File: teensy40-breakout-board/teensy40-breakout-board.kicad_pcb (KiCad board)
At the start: 2 copper layers, 18 x 56.1 mm, 3 parts, among them J1 Conn_01x08, J2 Conn_01x08, U1 Teensy4.0_WithBottomAndEdge

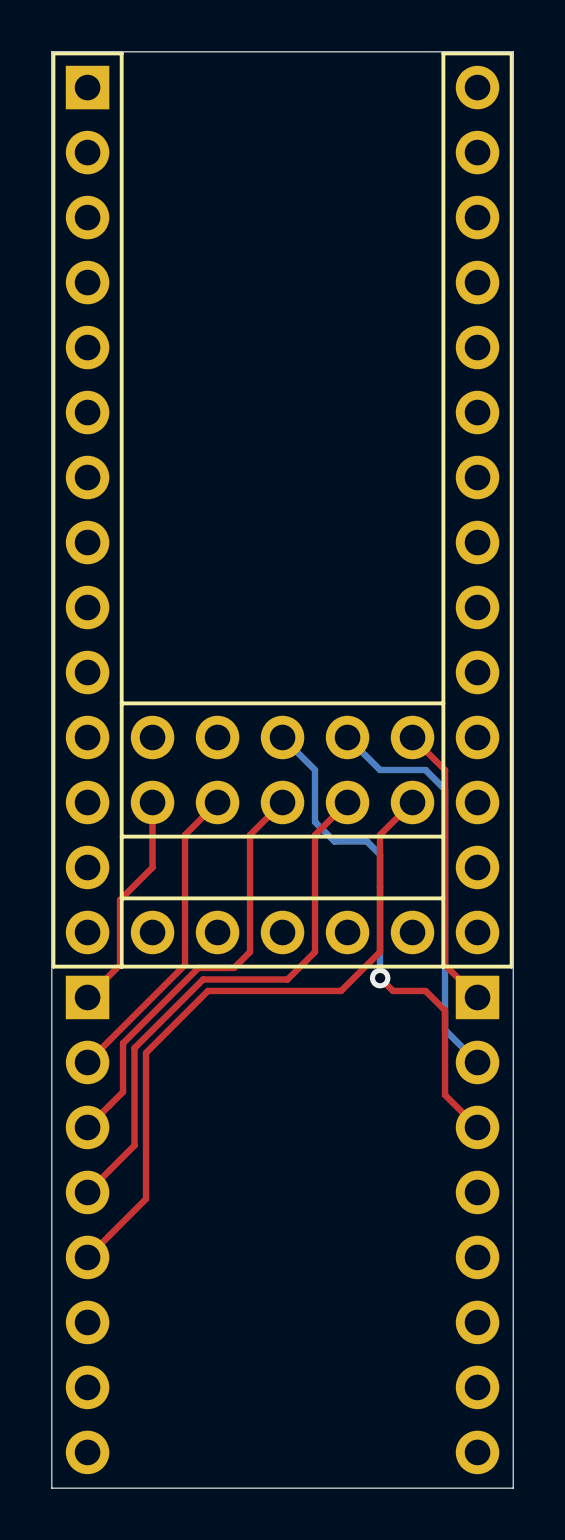
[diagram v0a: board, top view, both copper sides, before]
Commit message: Complete routing
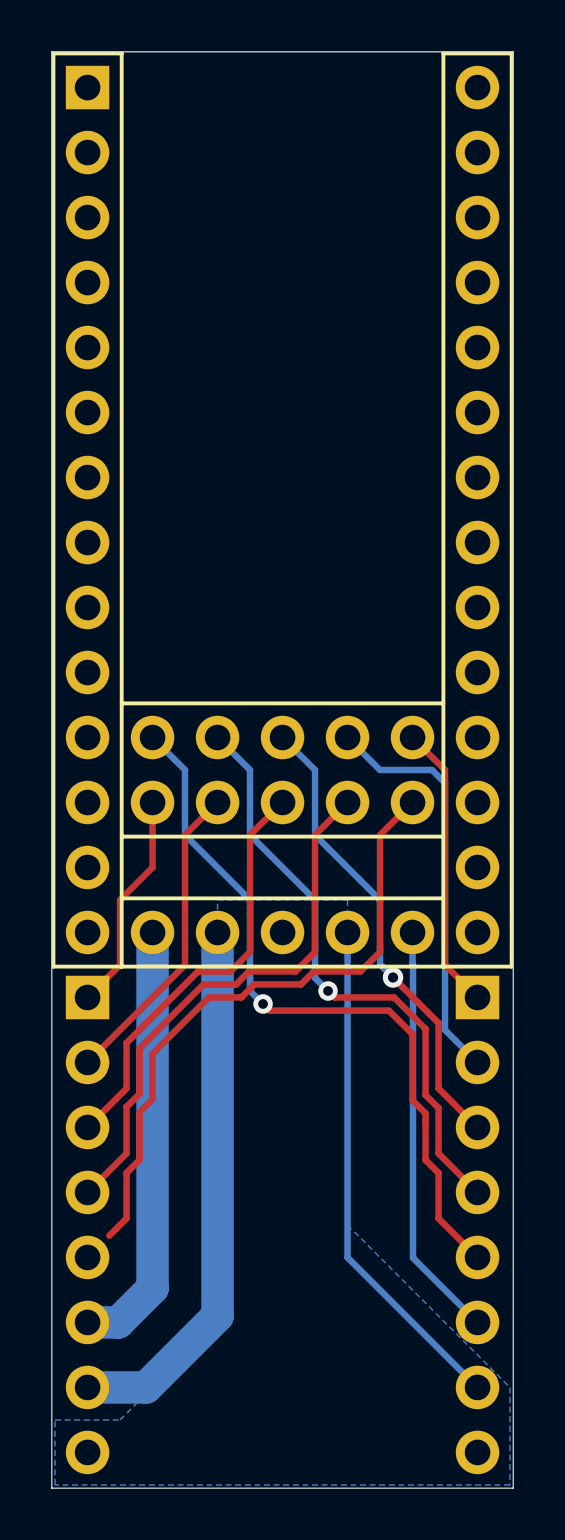
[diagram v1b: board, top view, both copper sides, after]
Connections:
- net Net-(J1-Pad6) renamed VCC
- net Net-(J1-Pad7) renamed +3V3
- net Net-(J1-Pad8) renamed GND
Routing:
- net Net-(J2-Pad5): track 0.00 -> 28.3 mm, vias 0 -> 1
- net Net-(J2-Pad4): track 0.00 -> 23.4 mm, vias 0 -> 1
- net +3V3: track 0.00 -> 21.2 mm
- net Net-(J2-Pad7): track 0.00 -> 19.9 mm
- net VCC: track 0.00 -> 17.0 mm
- net Net-(J2-Pad6): track 0.00 -> 16.3 mm
- net Net-(J2-Pad3): track 19.9 -> 18.4 mm
- net Net-(J1-Pad5): track 26.1 -> 24.7 mm
- added copper zone on B.Cu, net GND
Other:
- net class Default: clearance 0.2 -> 0.254; trace_width 0.25 -> 0.254; via_dia 0.8 -> 0.762; via_drill 0.4 -> 0.381
- net class Power added: clearance 0.254, trace_width 1.27, via_dia 1.524, via_drill 0.762
- rule trace_clearance: 0.2 -> 0.254
